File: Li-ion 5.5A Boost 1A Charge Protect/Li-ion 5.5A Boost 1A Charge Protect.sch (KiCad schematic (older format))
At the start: 58 parts, among them J1 USB_C_FEMALE, Q1 BUK6D30-40E, SW1 SW_DPST, U1 AP9101CK6, U2 ECH8695R-TL-W, U3 MCP73833T, U4 PAM2423AECADJR

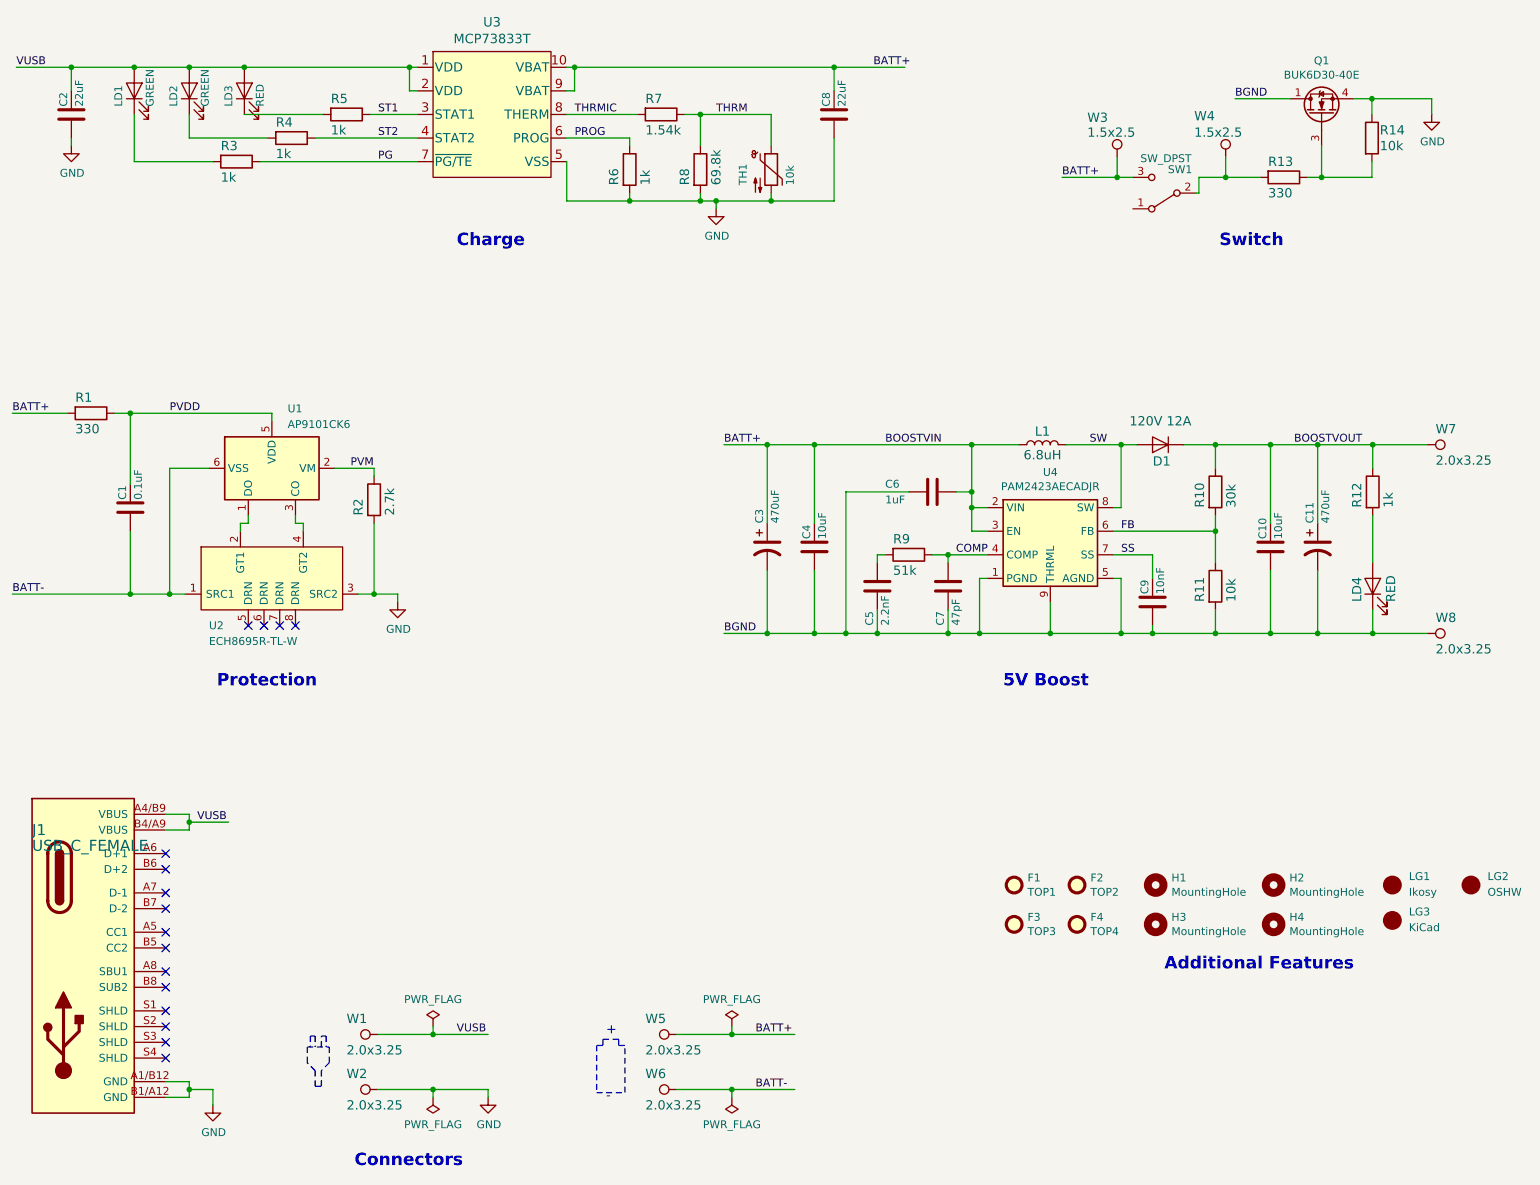
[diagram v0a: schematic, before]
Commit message: Component extraction
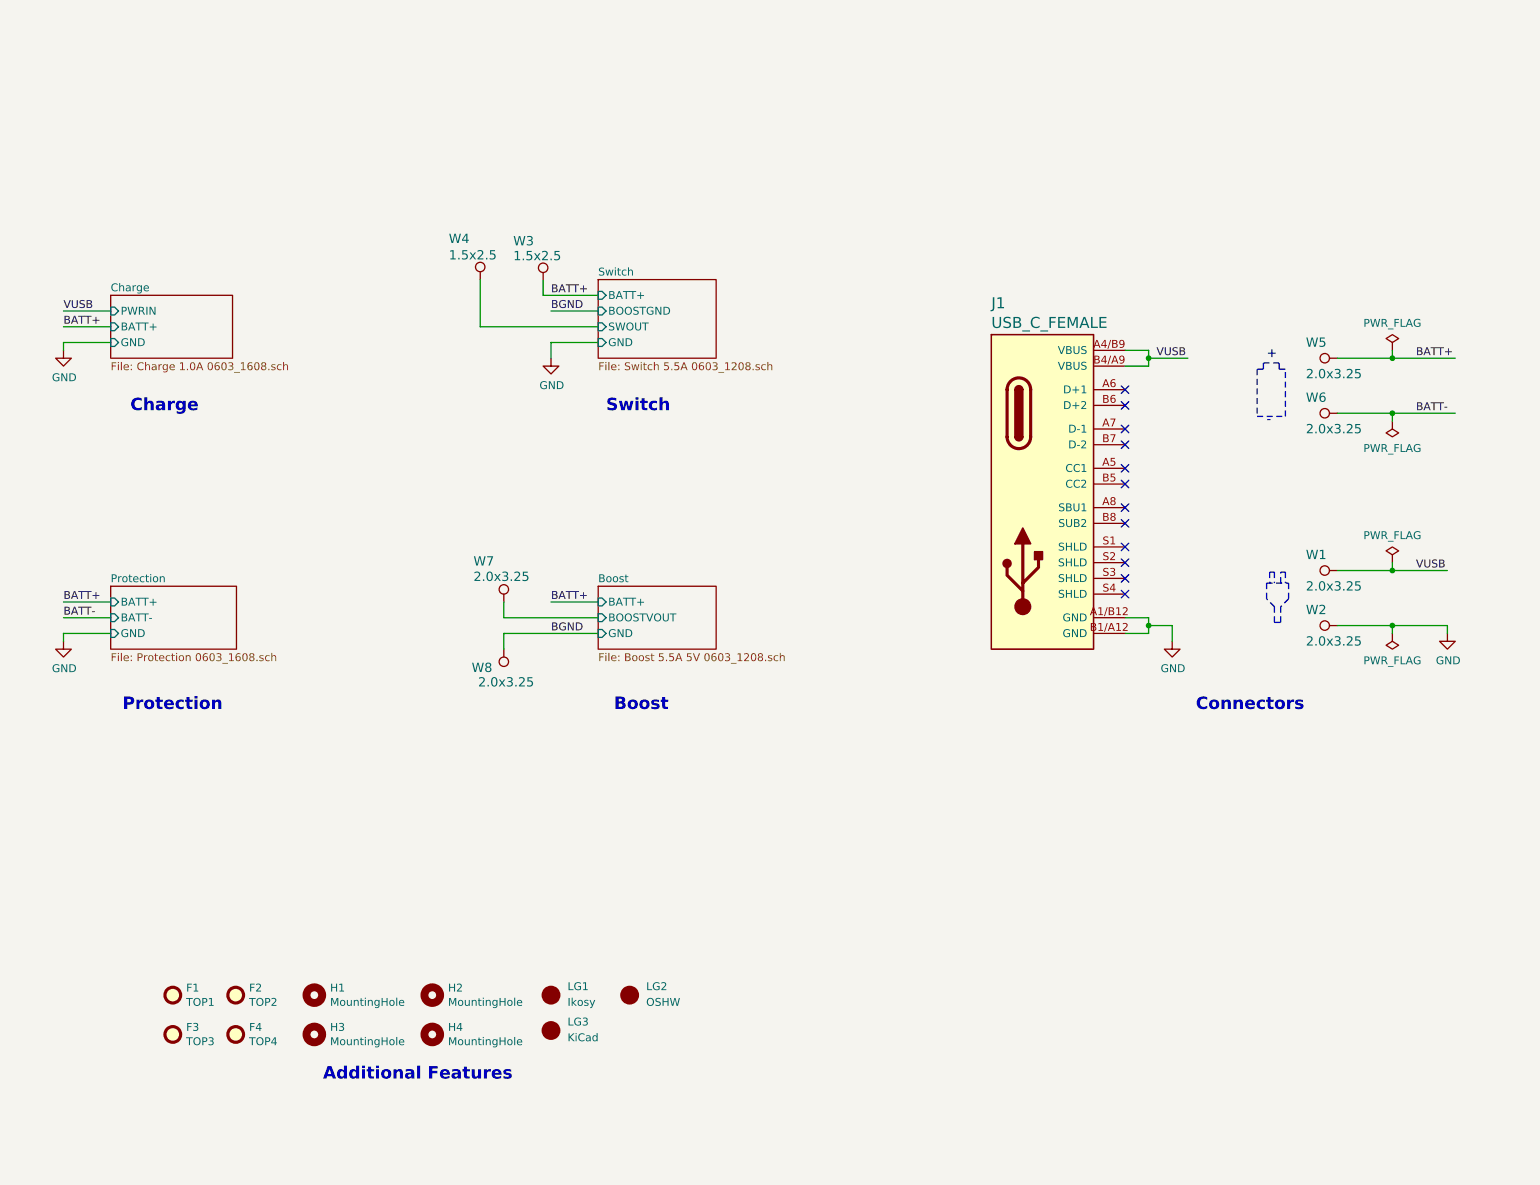
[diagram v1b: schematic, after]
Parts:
- removed C1: 0.1uF, Frequently_Used_LE:0603_1608Metric, symbol Frequently_Used_LE:C
- removed C10, C4: 10uF, Frequently_Used_LE:0603_1608Metric, symbol Frequently_Used_LE:C
- removed C11, C3: 470uF, Li_Ion_LE:CP_Elec_10x10.5, symbol Frequently_Used_LE:CP1
- removed C2, C8: 22uF, Frequently_Used_LE:0603_1608Metric, symbol Frequently_Used_LE:C
- removed C5: 2.2nF, Frequently_Used_LE:0603_1608Metric, symbol Frequently_Used_LE:C
- removed C6: 1uF, Frequently_Used_LE:0603_1608Metric, symbol Frequently_Used_LE:C
- removed C7: 47pF, Frequently_Used_LE:0603_1608Metric, symbol Frequently_Used_LE:C
- removed C9: 10nF, Frequently_Used_LE:0603_1608Metric, symbol Frequently_Used_LE:C
- removed D1: 120V 12A, Li_Ion_LE:NTS12120EMFST1G, symbol Li_Ion_LE:D_NTS12120EMFST1G
- removed L1: 6.8uH, Li_Ion_LE:L_MGV1004, symbol Frequently_Used_LE:L
- removed LD1, LD2: GREEN, Frequently_Used_LE:LED_0805_2012Metric, symbol Frequently_Used_LE:LED
- removed LD3, LD4: RED, Frequently_Used_LE:LED_0805_2012Metric, symbol Frequently_Used_LE:LED
- removed Q1: BUK6D30-40E, Li_Ion_LE:BUK6D3040EX, symbol Li_Ion_LE:BUK6D30-40E
- removed R1, R13: 330, Frequently_Used_LE:0603_1608Metric, symbol Frequently_Used_LE:R
- removed R10: 30k, Frequently_Used_LE:0603_1608Metric, symbol Frequently_Used_LE:R
- removed R11, R14: 10k, Frequently_Used_LE:0603_1608Metric, symbol Frequently_Used_LE:R
- removed R12, R3, R4, R5, R6: 1k, Frequently_Used_LE:0603_1608Metric, symbol Frequently_Used_LE:R
- removed R2: 2.7k, Frequently_Used_LE:0603_1608Metric, symbol Frequently_Used_LE:R
- removed R7: 1.54k, Frequently_Used_LE:0603_1608Metric, symbol Frequently_Used_LE:R
- removed R8: 69.8k, Frequently_Used_LE:0603_1608Metric, symbol Frequently_Used_LE:R
- removed R9: 51k, Frequently_Used_LE:0603_1608Metric, symbol Frequently_Used_LE:R
- removed SW1: SW_DPST, Button_Switch_LE:CL-SB-22A_Edge, symbol Button_Switch_LE:CL-SB-22A
- removed TH1: 10k, Frequently_Used_LE:0603_1608Metric, symbol Li_Ion_LE:Thermistor_NTC
- removed U1: AP9101CK6, Li_Ion_LE:SOT-23-6, symbol Li_Ion_LE:AP9101CK6
- removed U2: ECH8695R-TL-W, Li_Ion_LE:SOT65P280X95-8N, symbol Li_Ion_LE:ECH8695R-TL-W_Gates_on_Top
- removed U3: MCP73833T, Li_Ion_LE:MCP73833, symbol Li_Ion_LE:MCP73833T
- removed U4: PAM2423AECADJR, Li_Ion_LE:PAM2423AECADJR, symbol Li_Ion_LE:PAM2423AECADJR
- F1, F2, F3, F4, H1, H2, H3, H4, LG1, LG2, LG3, W1, W2, W3, W4, W5, W6, W7, W8: Source None -> (none); Source 1 (none) -> None; Source 1 Part No. (none) -> None; Source Part No. None -> (none)
- J1: Source Digikey -> (none); Source 1 (none) -> Digikey; Source 1 Part No. (none) -> 2073-USB4110-GF-A-1-ND; Source Part No. 2073-USB4110-GF-A-1-ND -> (none)
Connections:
- net labels removed: BOOSTVIN, BOOSTVOUT, COMP, FB, PG, PROG, PVDD, PVM, SS, ST1, ST2, SW, THRM, THRMIC
- wire segments 172 -> 44
- no-connect marks 16 -> 12
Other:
- note added: "Boost"
- note removed: "5V Boost"
- moved on the sheet: F1, F2, F3, F4, H1, H2, H3, H4, J1, LG1, LG2, LG3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
